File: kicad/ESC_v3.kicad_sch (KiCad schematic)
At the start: 64 parts, among them J1 Conn_01x07, J10 Conn_01x03, J2 Conn_01x05_Pin, J3 USB_C_Receptacle_USB2.0, J4 Conn_01x04, J6 Conn_01x06_Pin, J7 Conn_01x02_Pin, J8 Conn_01x04_Pin, J9 Conn_01x02, SW2 SW_Nidec_CAS-120A1, U1 STSPIN32G4, U10 BD4104, U14 MCP9700x-ETT, U2 AMS1117-5.0, X1 IQXO-70

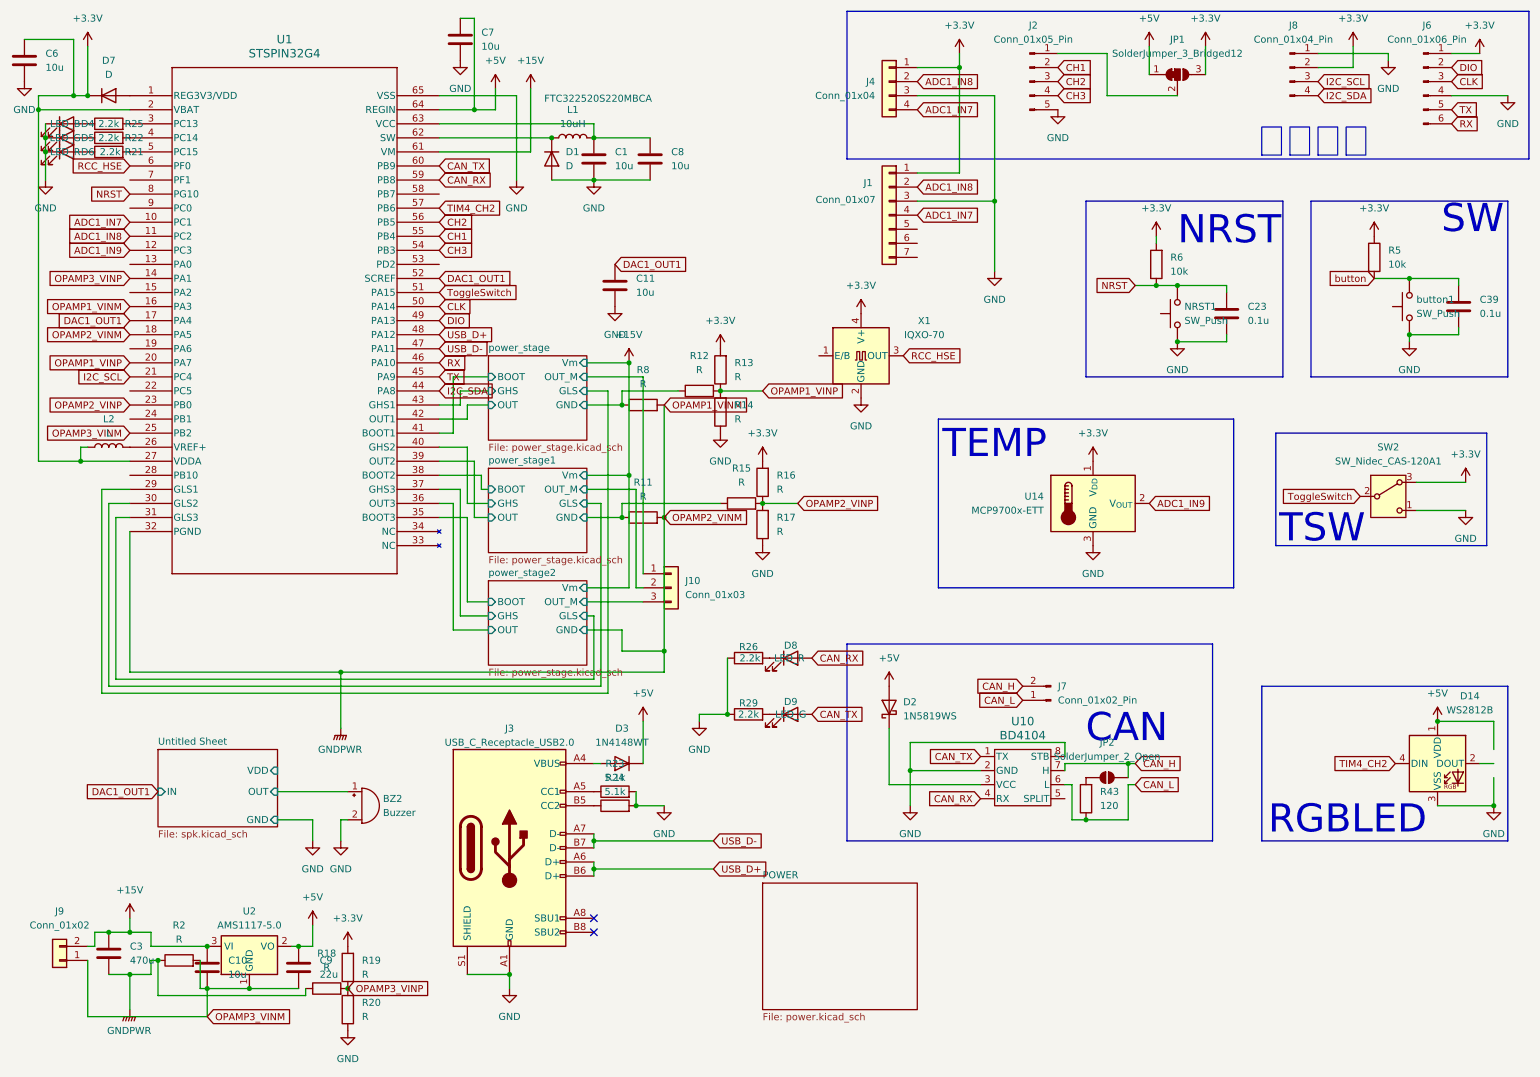
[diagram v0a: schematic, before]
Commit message: finish
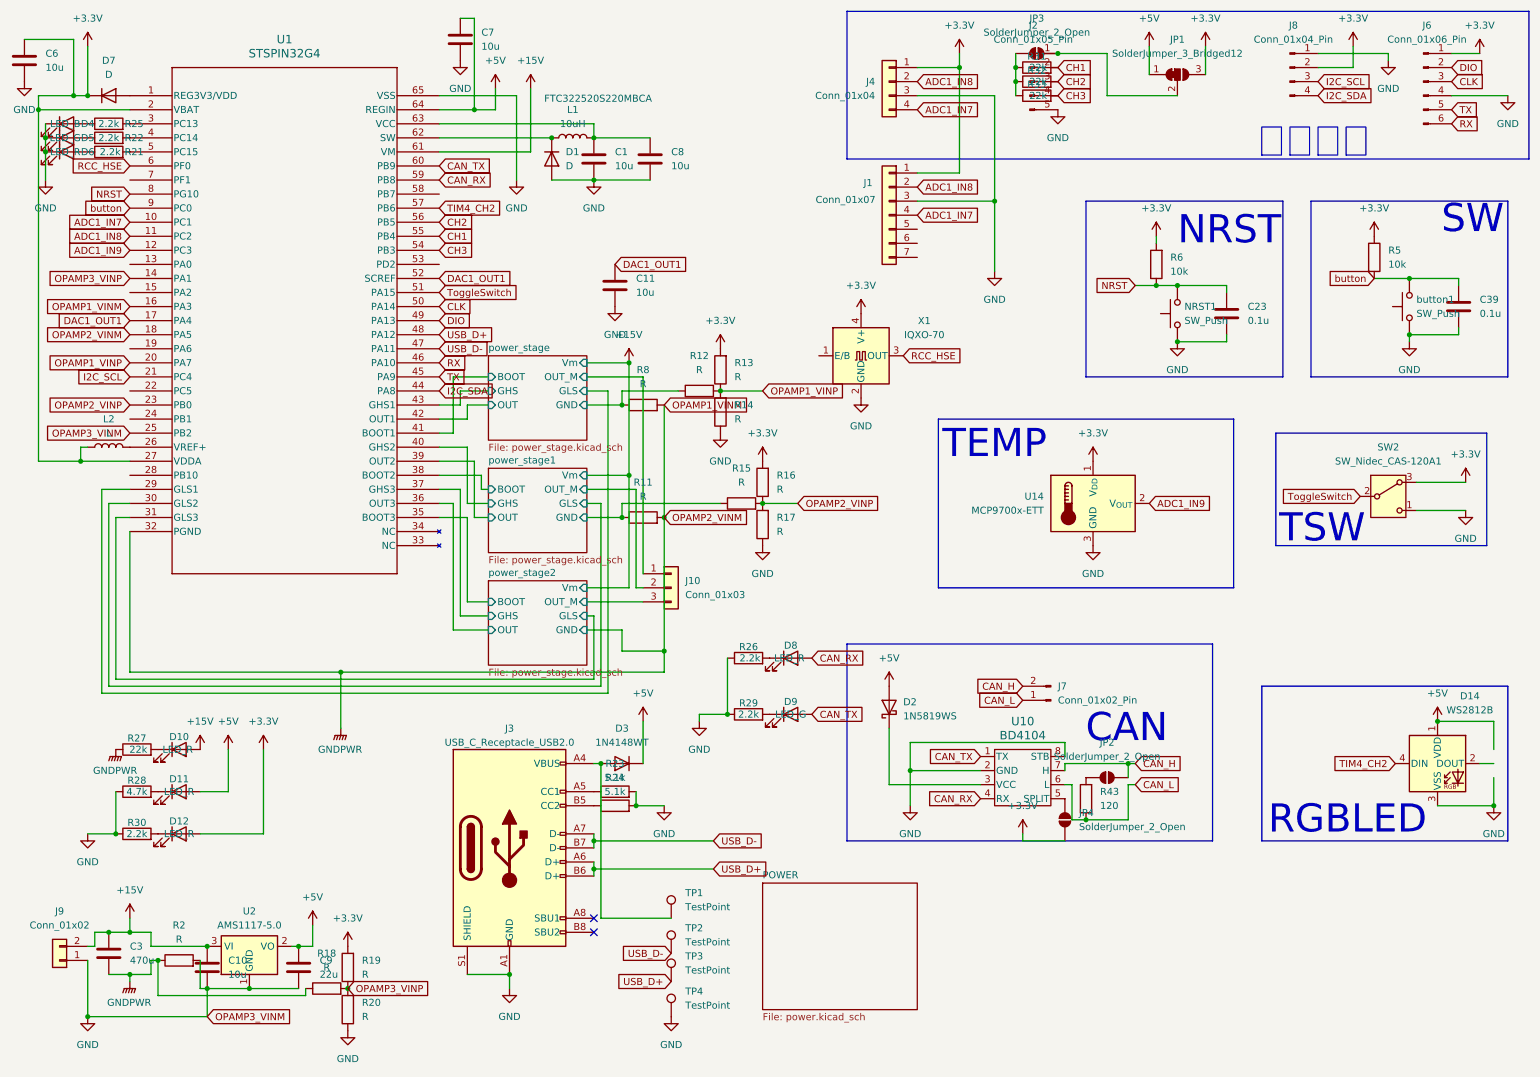
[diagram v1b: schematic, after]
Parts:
- removed BZ2: Buzzer, jisaku:buzzer_unified, symbol Device:Buzzer
- added D10, D11, D12: LED_R, LED_SMD:LED_0603_1608Metric, symbol Device:LED
- added JP3, JP4: SolderJumper_2_Open, Jumper:SolderJumper-2_P1.3mm_Open_RoundedPad1.0x1.5mm, symbol Jumper:SolderJumper_2_Open
- added R27, R31, R32, R33: 22k, Resistor_SMD:R_0402_1005Metric_Pad0.72x0.64mm_HandSolder, symbol Device:R
- added R28: 4.7k, Resistor_SMD:R_0402_1005Metric_Pad0.72x0.64mm_HandSolder, symbol Device:R
- added R30: 2.2k, Resistor_SMD:R_0402_1005Metric_Pad0.72x0.64mm_HandSolder, symbol Device:R
- added TP1, TP2, TP3, TP4: TestPoint, TestPoint:TestPoint_Pad_D1.5mm, symbol Connector:TestPoint
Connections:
- net OPAMP3_VINM is gone; now on net GND: C10.2, C9.2, J9.1 (Pin_1), R2.2, U1.25 (PB2), U2.1 (GND)
- net +15V: now also D10.2 (A)
- net +3.3V: now also D12.2 (A), JP4.1 (A)
- net +5V: now also D11.2 (A)
- net CH1: now also R31.2
- net CH2: now also R32.2
- net CH3: now also R33.2
- net GND: now also R28.1, R30.1, TP4.1
- net GNDPWR: now also R27.1
- net USB_D+: now also TP3.1
- net USB_D-: now also TP2.1
- net button: now also U1.9 (PC0)
- net at D3.2 (A), J3.A4 (VBUS), J3.A9 (VBUS)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: now also TP1.1
- net at J2.1 (Pin_1), JP1.2 (C): now also JP3.2 (B)
- net at U10.5 (SPLIT): now also JP4.2 (B)
- new net: D10.1 (K), R27.2
- new net: D11.1 (K), R28.2
- new net: D12.1 (K), R30.2
- new net: JP3.1 (A), R31.1, R32.1, R33.1
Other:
- removed sheet Untitled Sheet
